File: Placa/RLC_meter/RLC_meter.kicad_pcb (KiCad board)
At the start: 2 copper layers, 12 parts, among them J1 BAT, J2 BAT, Q1 IRF4905, Q2 IRF4905, U3 L7805, U4 LM358

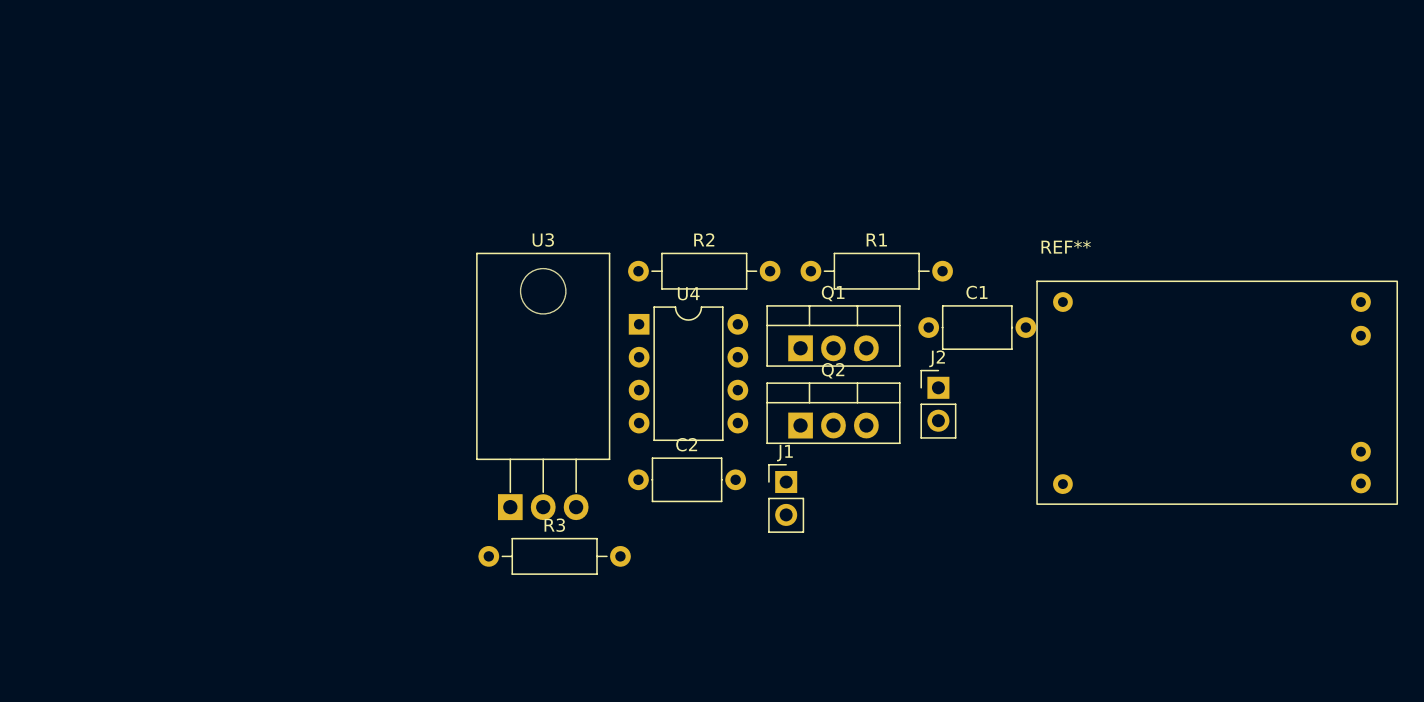
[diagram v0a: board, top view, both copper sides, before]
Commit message: massive update. Local to git
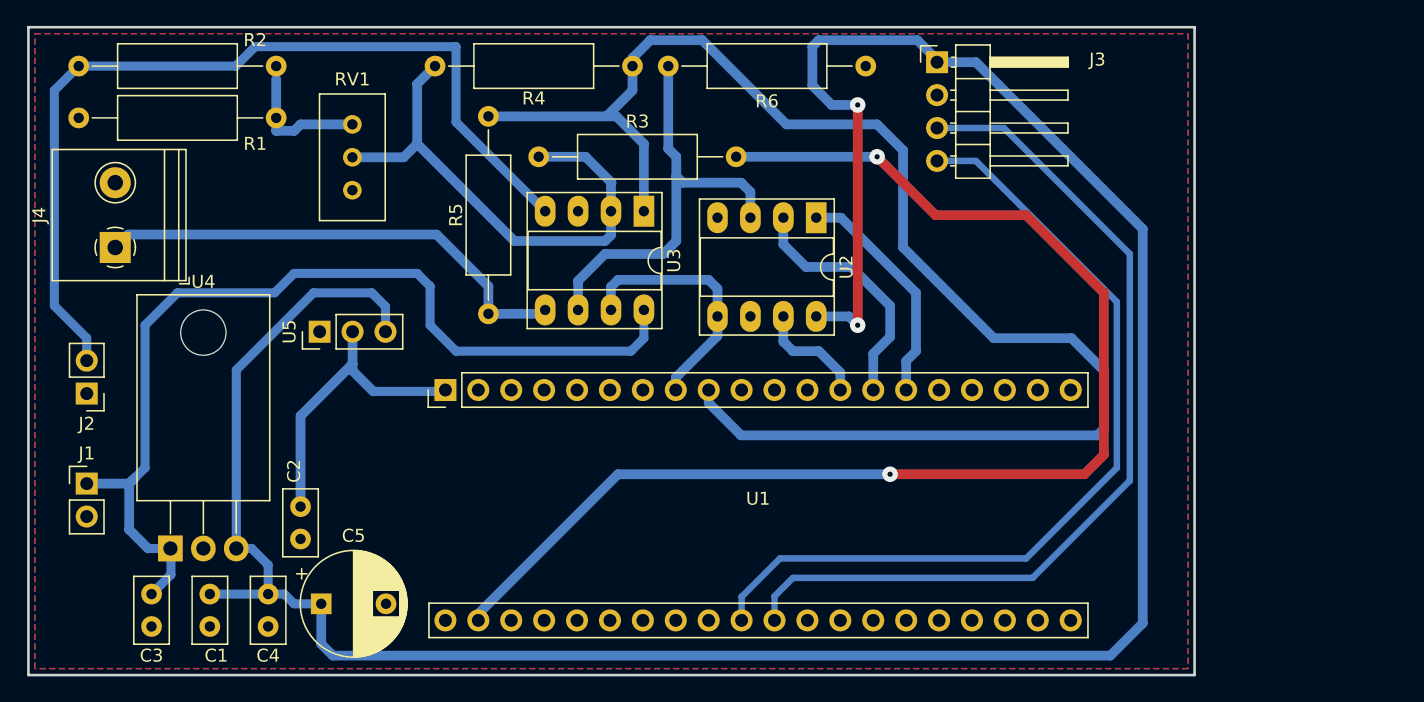
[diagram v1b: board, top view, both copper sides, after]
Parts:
- removed Q1, Q2: IRF4905, Package_TO_SOT_THT:TO-220-3_Vertical
- removed REF**: TP4056 module, RLC_meter:TP4056
- added C3: 100n, Capacitor_THT:C_Disc_D5.0mm_W2.5mm_P2.50mm, F.Cu at (34.0, 63.8)
- added C4: 100n, Capacitor_THT:C_Disc_D5.0mm_W2.5mm_P2.50mm, F.Cu at (43.0, 63.8)
- added C5: 100u, Capacitor_THT:CP_Radial_D8.0mm_P5.00mm, F.Cu at (47.1, 64.5)
- added J3: HC05, Connector_PinHeader_2.54mm:PinHeader_1x04_P2.54mm_Horizontal, F.Cu at (94.6, 22.7)
- added J4: Load_terminal, TerminalBlock_Philmore:TerminalBlock_Philmore_TB132_1x02_P5.00mm_Horizontal, F.Cu at (31.2, 37.0)
- added R4: 100k, Resistor_THT:R_Axial_DIN0309_L9.0mm_D3.2mm_P15.24mm_Horizontal, F.Cu at (55.9, 23.0)
- added R5: 560, Resistor_THT:R_Axial_DIN0309_L9.0mm_D3.2mm_P15.24mm_Horizontal, F.Cu at (60.0, 26.9)
- added R6: 560, Resistor_THT:R_Axial_DIN0309_L9.0mm_D3.2mm_P15.24mm_Horizontal, F.Cu at (89.1, 23.0)
- added RV1: 50k, Potentiometer_THT:Potentiometer_Bourns_3386C_Horizontal, F.Cu at (49.5, 27.5)
- added U1: LPC845, RLC_meter:LPC845, F.Cu at (80.8, 56.9)
- added U2: X9Cxxx, Package_DIP:DIP-8_W7.62mm_Socket_LongPads, F.Cu at (85.3, 34.7)
- added U5: AMS1117-3.3, Connector_PinHeader_2.54mm:PinHeader_1x03_P2.54mm_Vertical, F.Cu at (47.0, 43.5)
- C1, C2: value C -> 100n; footprint Capacitor_THT:C_Axial_L5.1mm_D3.1mm_P7.50mm_Horizontal -> Capacitor_THT:C_Disc_D5.0mm_W2.5mm_P2.50mm
- J1: value BAT -> Batt1
- J2: value BAT -> Batt2
- R1: value R -> 150k; footprint Resistor_THT:R_Axial_DIN0207_L6.3mm_D2.5mm_P10.16mm_Horizontal -> Resistor_THT:R_Axial_DIN0309_L9.0mm_D3.2mm_P15.24mm_Horizontal
- R2: value R -> 220k; footprint Resistor_THT:R_Axial_DIN0207_L6.3mm_D2.5mm_P10.16mm_Horizontal -> Resistor_THT:R_Axial_DIN0309_L9.0mm_D3.2mm_P15.24mm_Horizontal
- R3: value R -> 100k; footprint Resistor_THT:R_Axial_DIN0207_L6.3mm_D2.5mm_P10.16mm_Horizontal -> Resistor_THT:R_Axial_DIN0309_L9.0mm_D3.2mm_P15.24mm_Horizontal
- U3: value L7805 -> MC33202; footprint Package_TO_SOT_THT:TO-220-3_Horizontal_TabDown -> Package_DIP:DIP-8_W7.62mm_Socket_LongPads
- U4: value LM358 -> L7805; footprint Package_DIP:DIP-8_W7.62mm -> Package_TO_SOT_THT:TO-220-3_Horizontal_TabDown
- moved J2 65.7 mm to (29.0, 48.3), turned to 180 degrees
- moved C1 59.2 mm to (38.5, 63.8), turned to -90 degrees
- moved R1 57.7 mm to (28.4, 27.0)
- moved J1 54.0 mm to (29.0, 55.2)
- moved U4 40.1 mm to (35.5, 60.2)
- moved R2 32.1 mm to (43.6, 23.0), turned to 180 degrees
- moved R3 31.1 mm to (63.9, 30.0)
- moved C2 26.2 mm to (45.5, 57.0), turned to -90 degrees
- moved U3 25.1 mm to (72.0, 34.2), turned to -90 degrees
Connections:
- C1 pad 1: +BATT -> +5V
- C2 pad 1: VCC -> +3.3V
- J1 pad 1: Net-(J1-Pad1) -> +BATT
- J1 pad 2: /in_BAT2- -> GND
- J2 pad 1: Net-(J2-Pad1) -> GND
- J2 pad 2: /in_BAT1- -> -BATT
- R2 pad 2: /Signal_o -> -BATT
- R3 pad 1: /Singal_i -> Net-(R3-Pad1)
- R3 pad 2: /Signal_o -> /V_DAC
- U3 pad 1: +BATT -> /Signal_i
- U3 pad 2: GND -> Net-(R3-Pad1)
- U3 pad 3: VCC -> GND
- U4 pad 1: /Signal_o -> +BATT
- U4 pad 2: Net-(R1-Pad2) -> GND
- U4 pad 3: /DAC -> +5V
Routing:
- net +5V: track 0.00 -> 202.0 mm, vias 0 -> 2
- net /Signal_i: track 0.00 -> 112.6 mm
- net /V_DAC: track 0.00 -> 99.1 mm, vias 0 -> 2
- net +BATT: track 0.00 -> 73.5 mm
- net -BATT: track 0.00 -> 69.8 mm
- net /RX: track 0.00 -> 69.4 mm
- net /TX: track 0.00 -> 66.1 mm
- net Net-(R3-Pad1): track 0.00 -> 40.8 mm
- net /generated_signal: track 0.00 -> 37.5 mm
- net /POT+: track 0.00 -> 33.1 mm
- net +3.3V: track 0.00 -> 23.6 mm
- net /POT_V: track 0.00 -> 19.7 mm
- net /POT_U/D: track 0.00 -> 19.3 mm
- net /POT_INC: track 0.00 -> 17.9 mm
- net Net-(R1-Pad2): track 0.00 -> 10.1 mm
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- added copper zone on B.Cu, net GND
- added copper zone on F.Cu, net GND
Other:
- board outline added: 90 x 50 mm
